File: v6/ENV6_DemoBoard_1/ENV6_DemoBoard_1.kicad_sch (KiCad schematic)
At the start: 0 parts

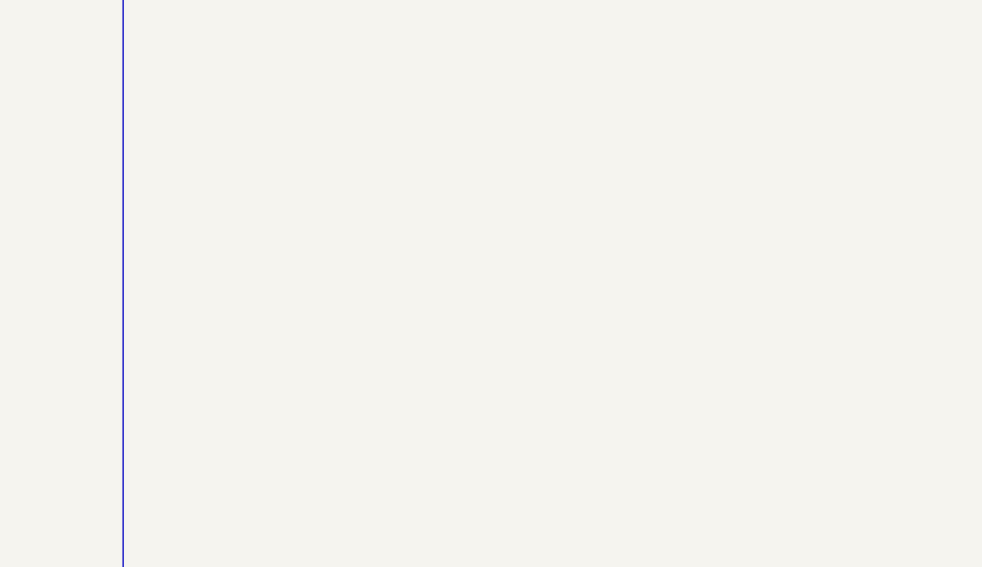
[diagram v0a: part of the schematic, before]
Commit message: First review of base module done
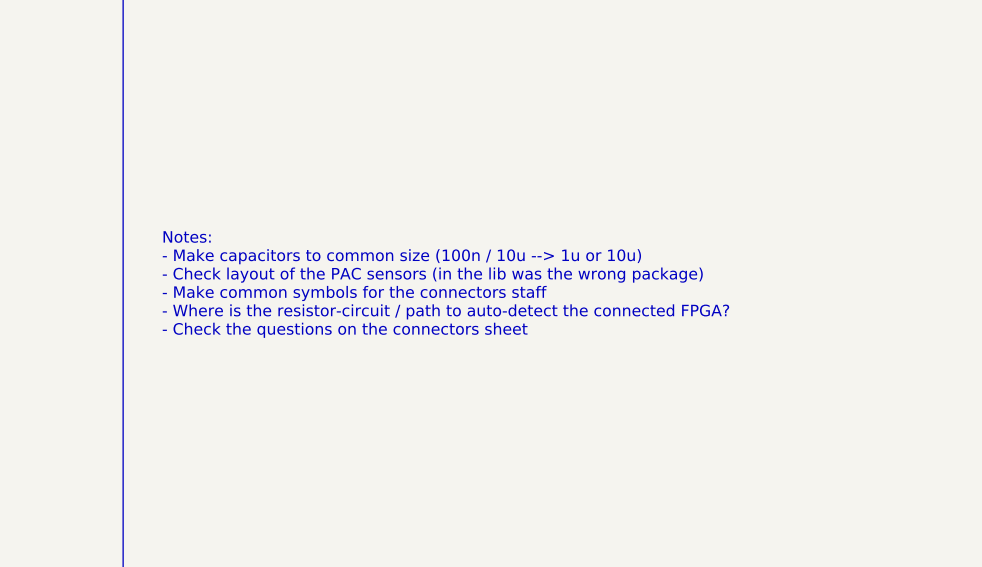
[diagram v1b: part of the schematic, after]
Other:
- note added: "Notes: - Make capacitors to common size (100n / 10u --> 1u or 10u) - Check layout of the PAC sensors (in the lib was the wrong package) - Make common symbols for the connectors staff - Where is the resistor-circuit / path to auto-detect the connected FPGA? - Check the questions on the connectors sheet"
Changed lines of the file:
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@@
+		)
+	)
+	(text "Notes:\n- Make capacitors to common size (100n / 10u --> 1u or 10u)\n- Check layout of the PAC sensors (in the lib was the wrong package)\n- Make common symbols for the connectors staff\n- Where is the resistor-circuit / path to auto-detect the connected FPGA?\n- Check the questions on the connectors sheet"
+		(exclude_from_sim no)
+		(at 179.578 163.83 0)
+		(effects
+			(font
+				(size 1.27 1.27)
+			)
+			(justify left bottom)
 		)
 	)
